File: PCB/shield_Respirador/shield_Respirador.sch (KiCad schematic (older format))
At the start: 30 parts, among them P1 Digital, P10 CONN_01X01, P11 CONN_01X01, P12 CONN_01X01, P13 CONN_01X01, P2 Power, P3 Analog, P4 Analog, P5 PWM, P6 PWM, P7 Communication, P8 CONN_01X01, P9 CONN_01X01

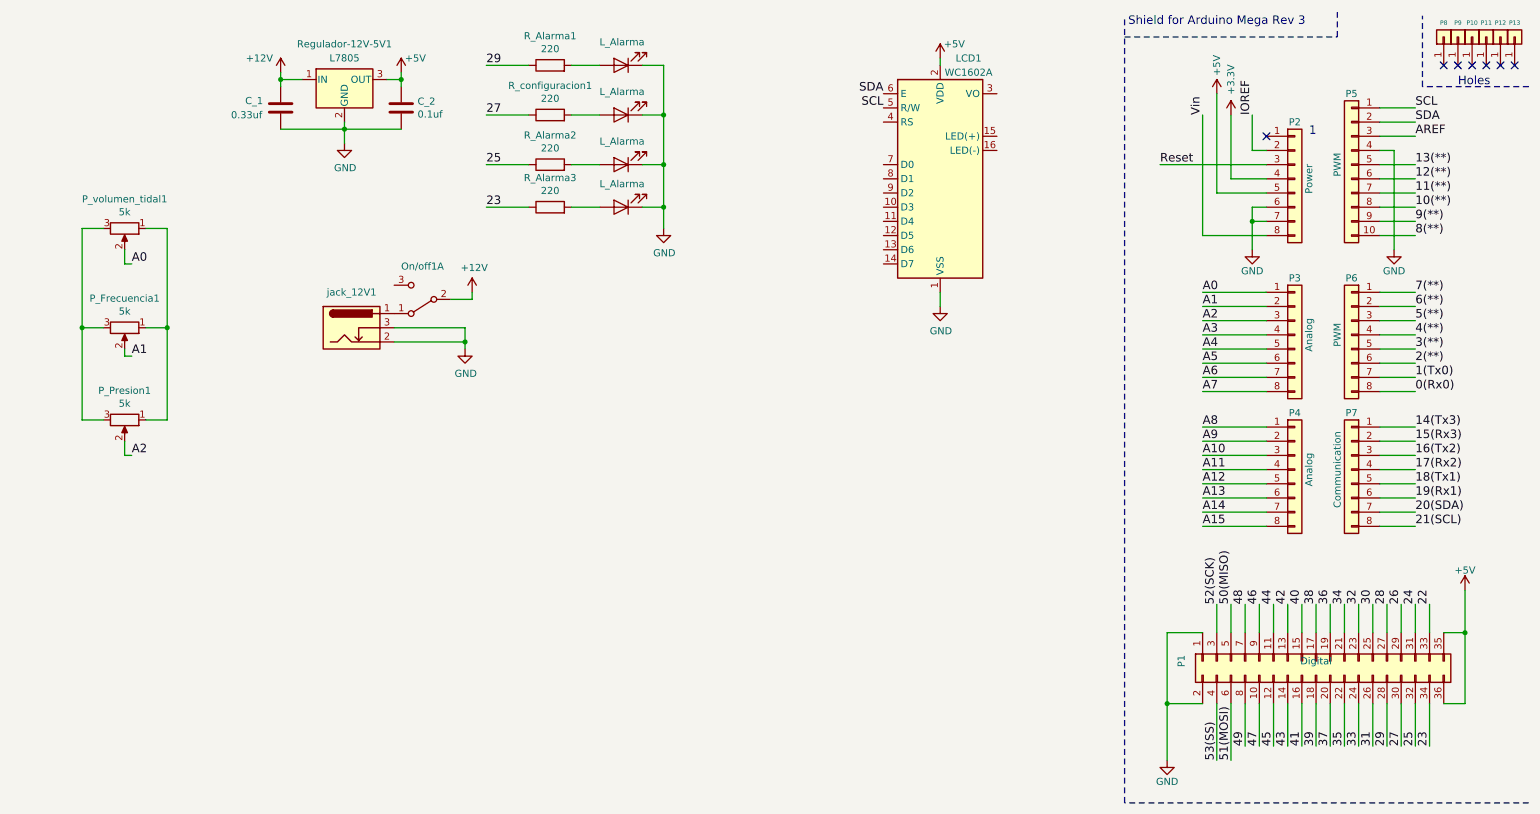
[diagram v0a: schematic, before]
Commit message: version 0.4
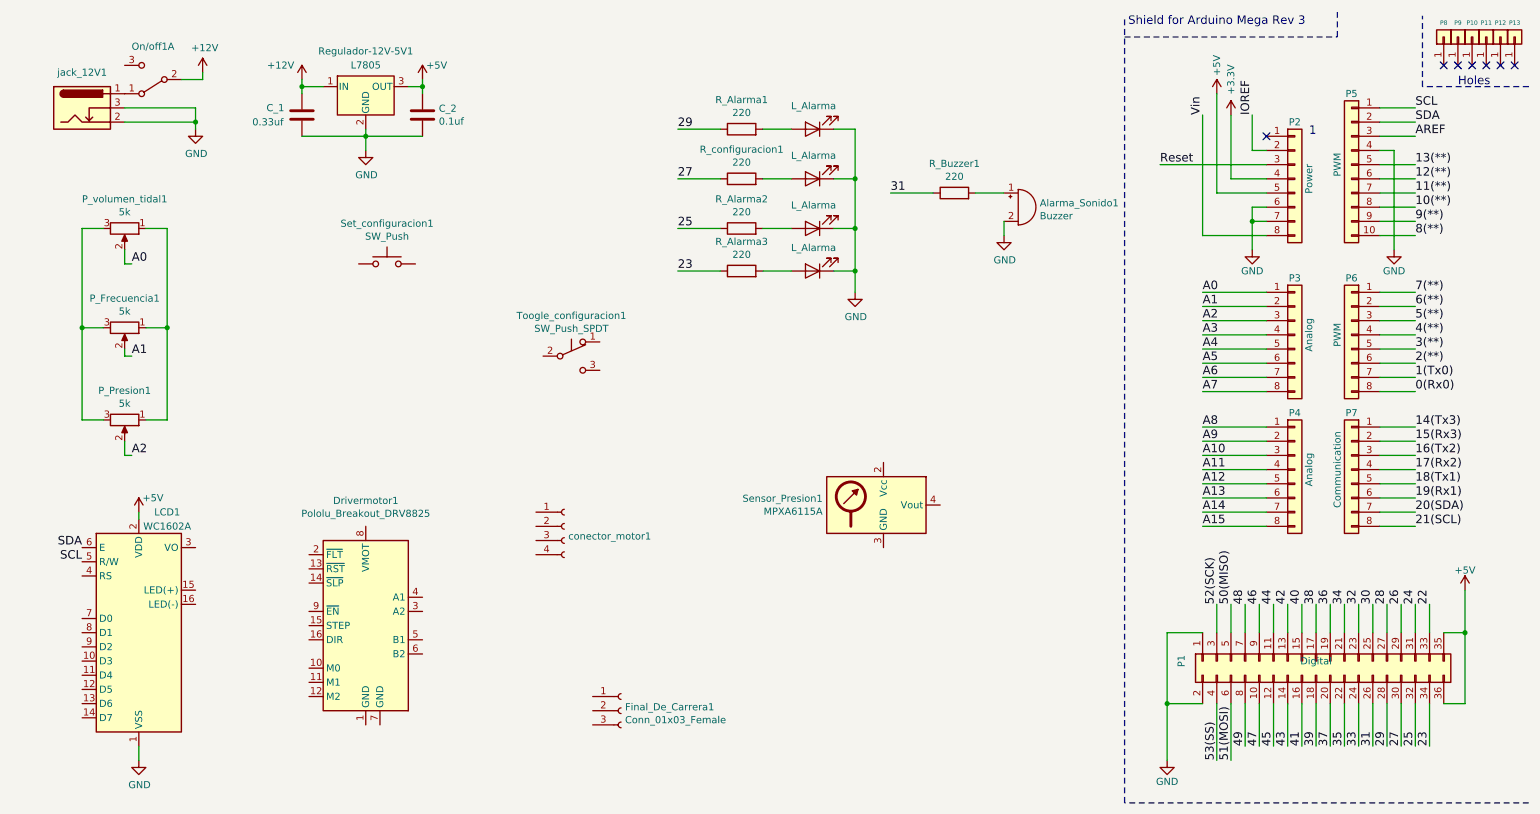
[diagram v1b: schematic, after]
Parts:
- added Alarma_Sonido1: Buzzer, Buzzer_Beeper:MagneticBuzzer_ProSignal_ABI-009-RC, symbol Device:Buzzer
- added Drivermotor1: Pololu_Breakout_DRV8825, Module:Pololu_Breakout-16_15.2x20.3mm, symbol Driver_Motor:Pololu_Breakout_DRV8825
- added Final_De_Carrera1: Conn_01x03_Female, Connector_PinSocket_2.00mm:PinSocket_1x03_P2.00mm_Vertical, symbol Connector:Conn_01x03_Female
- added R_Buzzer1: 220, Resistor_THT:R_Axial_DIN0207_L6.3mm_D2.5mm_P10.16mm_Horizontal, symbol Device:R
- added Sensor_Presion1: MPXA6115A, Package_DIP:DIP-8_W7.62mm_LongPads, symbol Sensor_Pressure:MPXA6115A
- added Set_configuracion1: SW_Push, TerminalBlock:TerminalBlock_bornier-2_P5.08mm, symbol Switch:SW_Push
- added Toogle_configuracion1: SW_Push_SPDT, TerminalBlock:TerminalBlock_bornier-3_P5.08mm, symbol Switch:SW_Push_SPDT
- added conector_motor1: Conn_01x04_Female, Connector_PinSocket_2.00mm:PinSocket_1x04_P2.00mm_Vertical, symbol Connector:Conn_01x04_Female
- On/off1: footprint Connector:Banana_Jack_3Pin -> TerminalBlock:TerminalBlock_bornier-3_P5.08mm
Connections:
- net 31: now also R_Buzzer1.1
- net GND: now also Alarma_Sonido1.2 (+)
- new net: Alarma_Sonido1.1 (-), R_Buzzer1.2
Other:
- moved on the sheet: C_1, C_2, LCD1, On/off1A, R_Alarma1, R_Alarma2, R_Alarma3, R_configuracion1, Regulador-12V-5V1, jack_12V1

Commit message: version 0.41 Esquematico terminado y irganizado
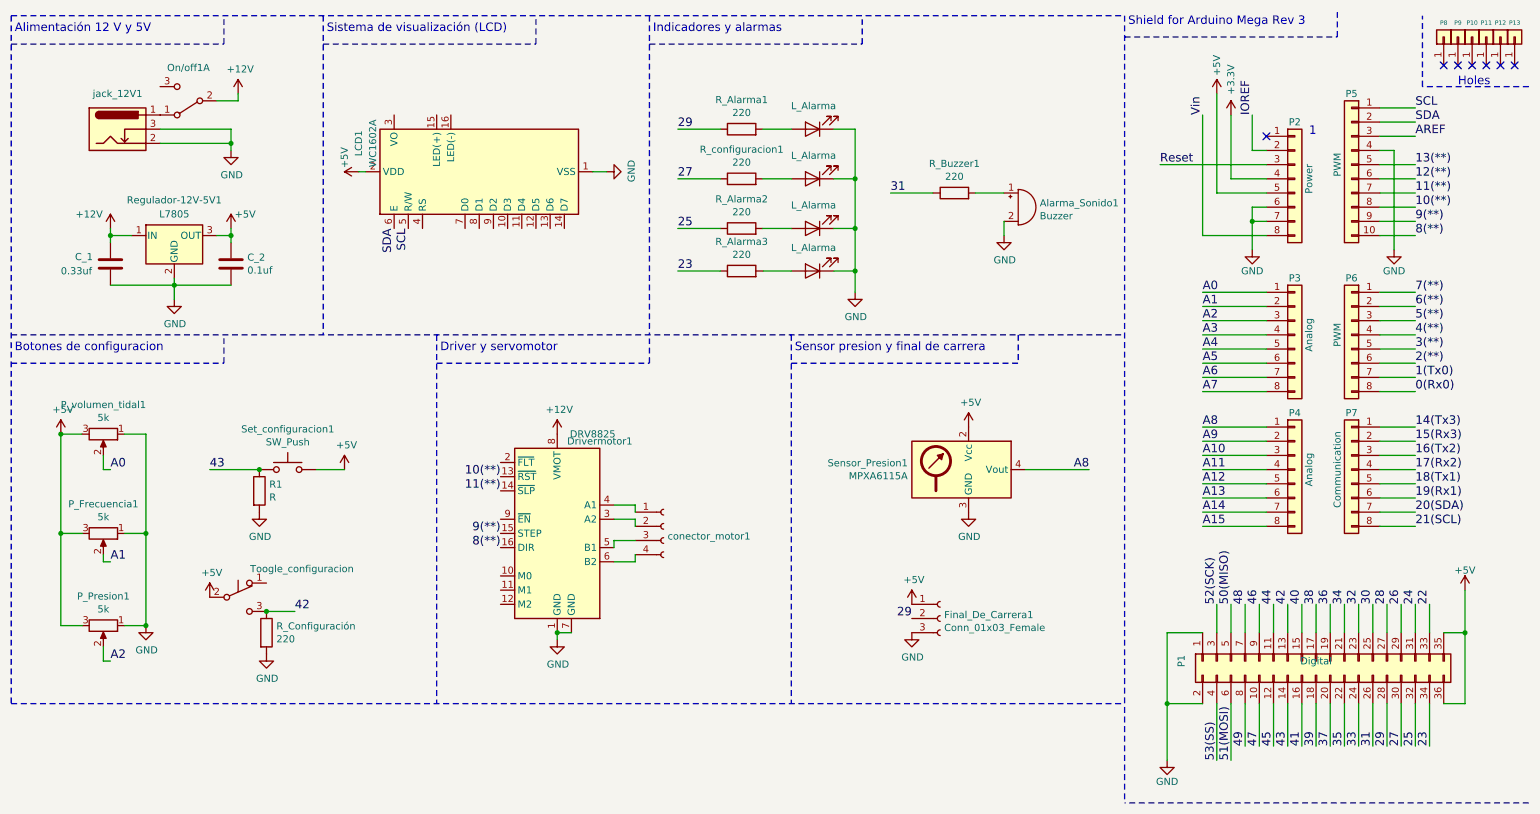
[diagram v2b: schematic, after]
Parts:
- added R1: R, symbol Device:R
- added R_Configuración: 220, symbol Device:R
- Drivermotor1: value Pololu_Breakout_DRV8825 -> DRV8825
- renumbered Toogle_configuracion1 to Toogle_configuracion
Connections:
- net +12V: now also Drivermotor1.8 (VMOT)
- net +5V: now also Final_De_Carrera1.1 (Pin_1), P_Frecuencia1.3, P_Presion1.3, P_volumen_tidal1.3, Sensor_Presion1.2 (Vcc), Set_configuracion1.2, Toogle_configuracion.2 (B)
- net 10(**): now also Drivermotor1.13 (~RST)
- net 11(**): now also Drivermotor1.14 (~SLP)
- net 29: now also Final_De_Carrera1.2 (Pin_2)
- net 42: now also Toogle_configuracion.3 (C), R_Configuración.1
- net 43: now also Set_configuracion1.1, R1.1
- net 8(**): now also Drivermotor1.16 (DIR)
- net 9(**): now also Drivermotor1.15 (STEP)
- net A8: now also Sensor_Presion1.4 (Vout)
- net GND: now also Drivermotor1.1 (GND), Drivermotor1.7 (GND), Final_De_Carrera1.3 (Pin_3), P_Frecuencia1.1, P_Presion1.1, P_volumen_tidal1.1, Sensor_Presion1.3 (GND), R1.2, R_Configuración.2
- net at Drivermotor1.3 (A2): now also conector_motor1.2 (Pin_2)
- net at Drivermotor1.4 (A1): now also conector_motor1.1 (Pin_1)
- net at Drivermotor1.5 (B1): now also conector_motor1.3 (Pin_3)
- net at Drivermotor1.6 (B2): now also conector_motor1.4 (Pin_4)
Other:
- note added: "Alimentación 12 V y 5V\n"
- note added: "Botones de configuracion\n"
- note added: "Driver y servomotor\n"
- note added: "Indicadores y alarmas"
- note added: "Sensor presion y final de carrera\n"
- note added: "Sistema de visualización (LCD)\n"
- moved on the sheet: C_1, C_2, Drivermotor1, Final_De_Carrera1, LCD1, On/off1A, P_Frecuencia1, P_Presion1, P_volumen_tidal1, Regulador-12V-5V1, Sensor_Presion1, Set_configuracion1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
